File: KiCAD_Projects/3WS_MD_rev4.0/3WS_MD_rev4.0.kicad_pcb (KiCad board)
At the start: 2 copper layers, 76 x 93 mm, 139 parts, among them P1 CONN_01X01, P11 TST, P12 TST, P13 CONN_01X06, P14 CONN_01X02, P15 CONN_01X02, P16 CONN_01X04, P17 CONN_01X04, P18 CONN_01X04, P19 CONN_01X04, P2 CONN_01X01, P20 CONN_01X06, P3 CONN_01X04, P4 CONN_02X02, P5 TST, P6 CONN_01X04, P7 CONN_01X02, P8 CONN_01X04, P9 TST, Q1 MOSFET_N, Q2 MOSFET_N, Q3 MOSFET_N, Q4 MOSFET_N, Q5 MOSFET_N, Q6 MOSFET_N, Q7 MOSFET_N, Q8 MOSFET_N, Q9 MOSFET_N, SW1 SW_PUSH, SW2 SW_PUSH, SW3 SW_PUSH, U1 STM32F103_48, U10 NCP1117ST33T3G, U2 SI8234, U3 SI8234, U4 LM7812, U5 SI8234, U6 SI8234, U7 NCP1117ST33T3G, U8 MAX3051, U9 SW_ROTARY_16, X2 CRYSTAL

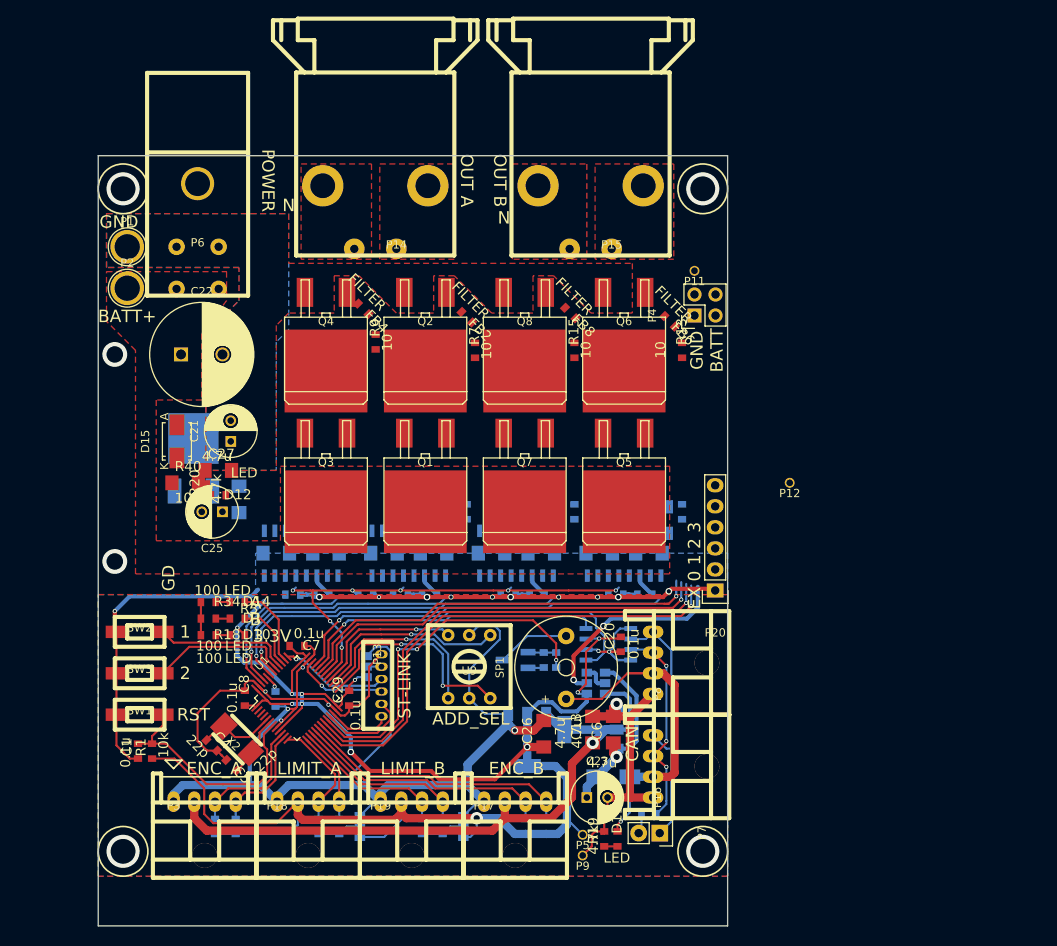
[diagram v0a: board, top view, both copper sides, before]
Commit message: no message
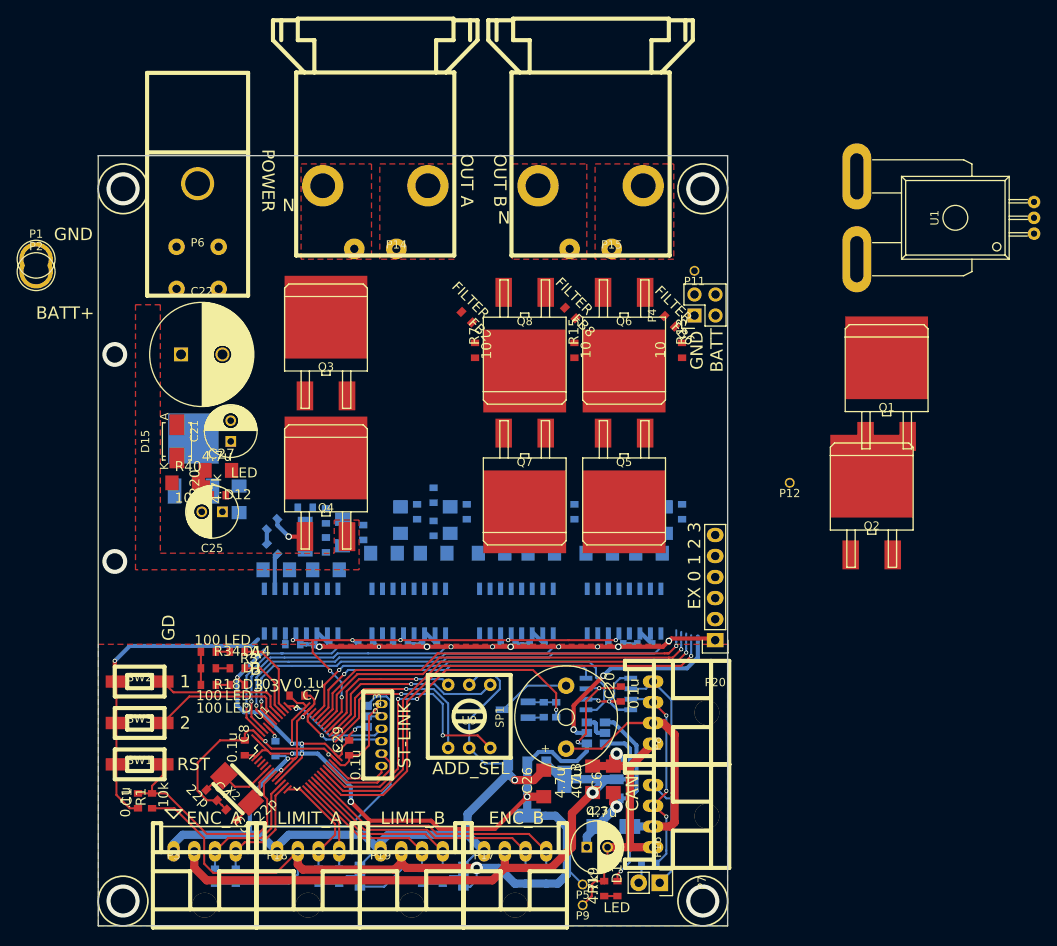
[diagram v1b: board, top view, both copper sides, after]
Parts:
- added U1: ACS758, RP_KiCAD_Libs:ACS785xCB, F.Cu at (113.0, 7.50)
- FB4, R9: moved to B.Cu
- moved Q2 59.7 mm to (93.4, 45.2), turned to 0 degrees
- moved Q1 56.0 mm to (95.2, 30.9), turned to 0 degrees
- moved FB4 28.2 mm to (21.0, 44.5), turned to 45 degrees
- moved R9 28.0 mm to (21.0, 47.5), turned to 315 degrees
- moved Q4 23.5 mm to (27.5, 43.0), turned to 0 degrees
- moved P2 11.2 mm to (-7.50, 14.0)
- moved P1 11.1 mm to (-7.50, 12.5)
- moved Q3 10.5 mm to (27.5, 26.0), turned to 0 degrees
- moved U2 7.00 mm to (37.5, 55.0)
- moved U3 7.00 mm to (24.5, 55.0)
- moved U5 7.00 mm to (63.5, 55.0)
- moved U6 7.00 mm to (50.5, 55.0)
- moved Q9 6.00 mm to (50.4, 66.9)
- moved R32 6.00 mm to (55.3, 66.9)
- moved R33 6.00 mm to (53.8, 66.9)
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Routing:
- net Net-(FB4-Pad2): track 0.00 -> 4.66 mm, vias 0 -> 1
- net Net-(R9-Pad2): track 0.00 -> 4.29 mm
- net Net-(FB4-Pad1): track 0.00 -> 1.73 mm
- net GNDPWR: track 1.00 -> 0.00 mm
- removed copper zone on F.Cu, net +BATT
- removed copper zone on B.Cu, net GND
- removed copper zone on B.Cu, net GNDPWR
